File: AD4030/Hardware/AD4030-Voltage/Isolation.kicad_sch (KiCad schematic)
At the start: 23 parts, among them J401 Conn_01x08, J402 Conn_01x10, U401 ADuM260N, U402 ADuM260N

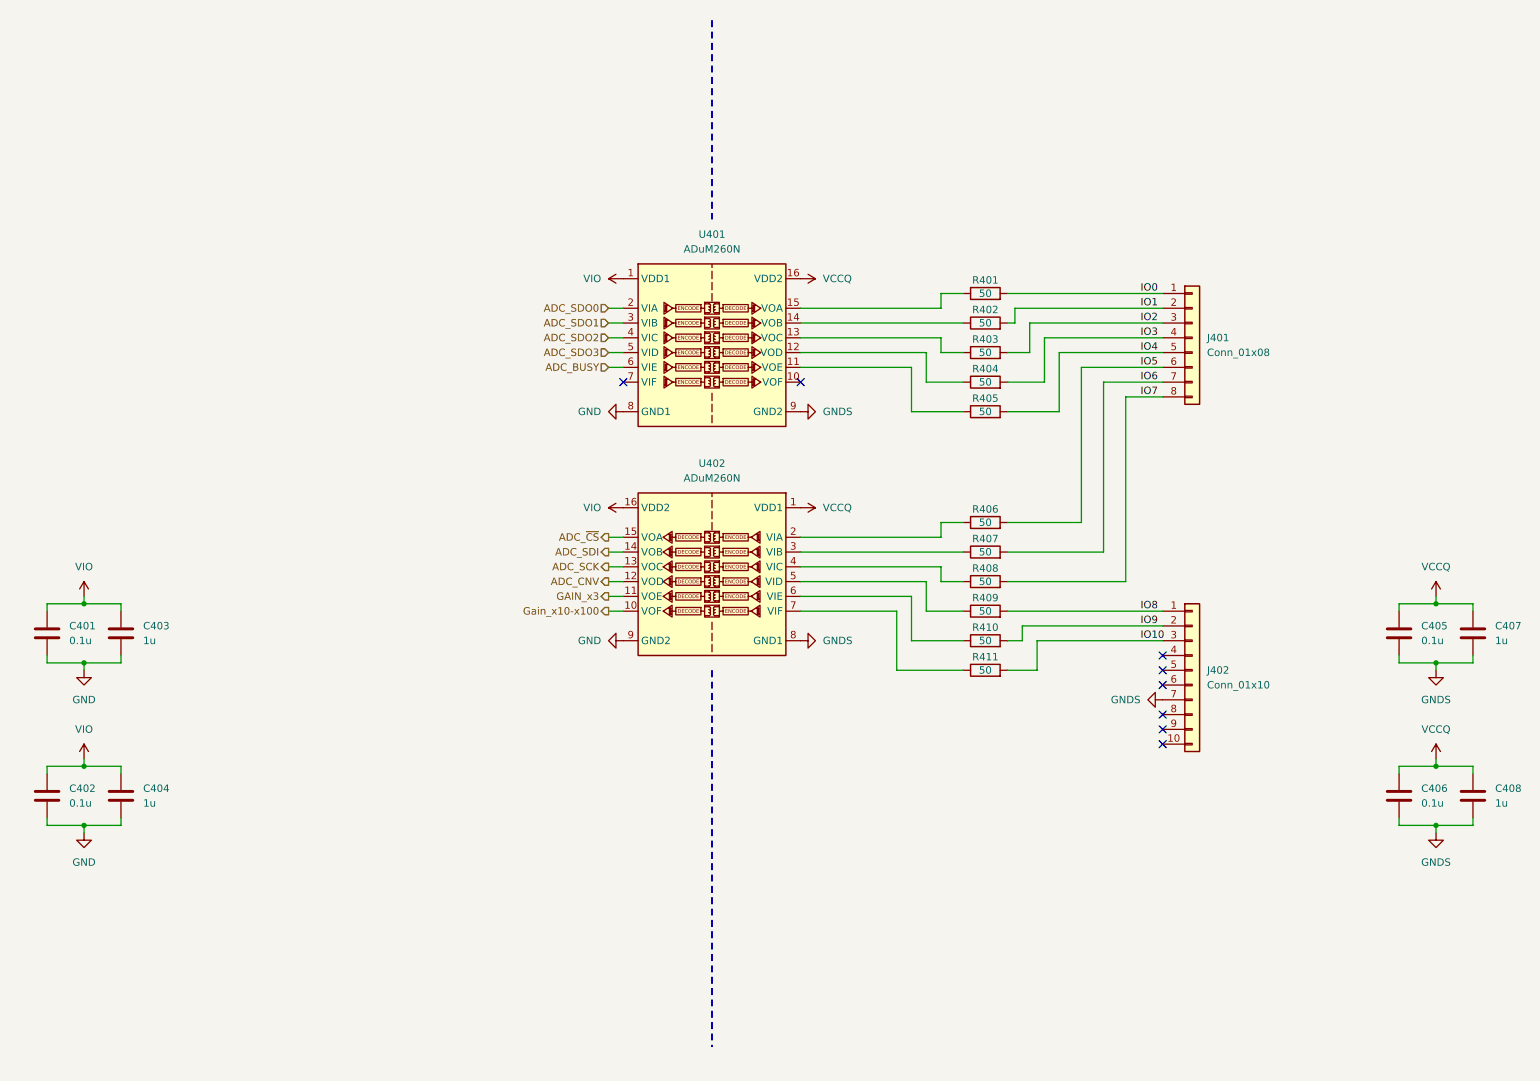
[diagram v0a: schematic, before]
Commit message: Hardware and started to create simulation.
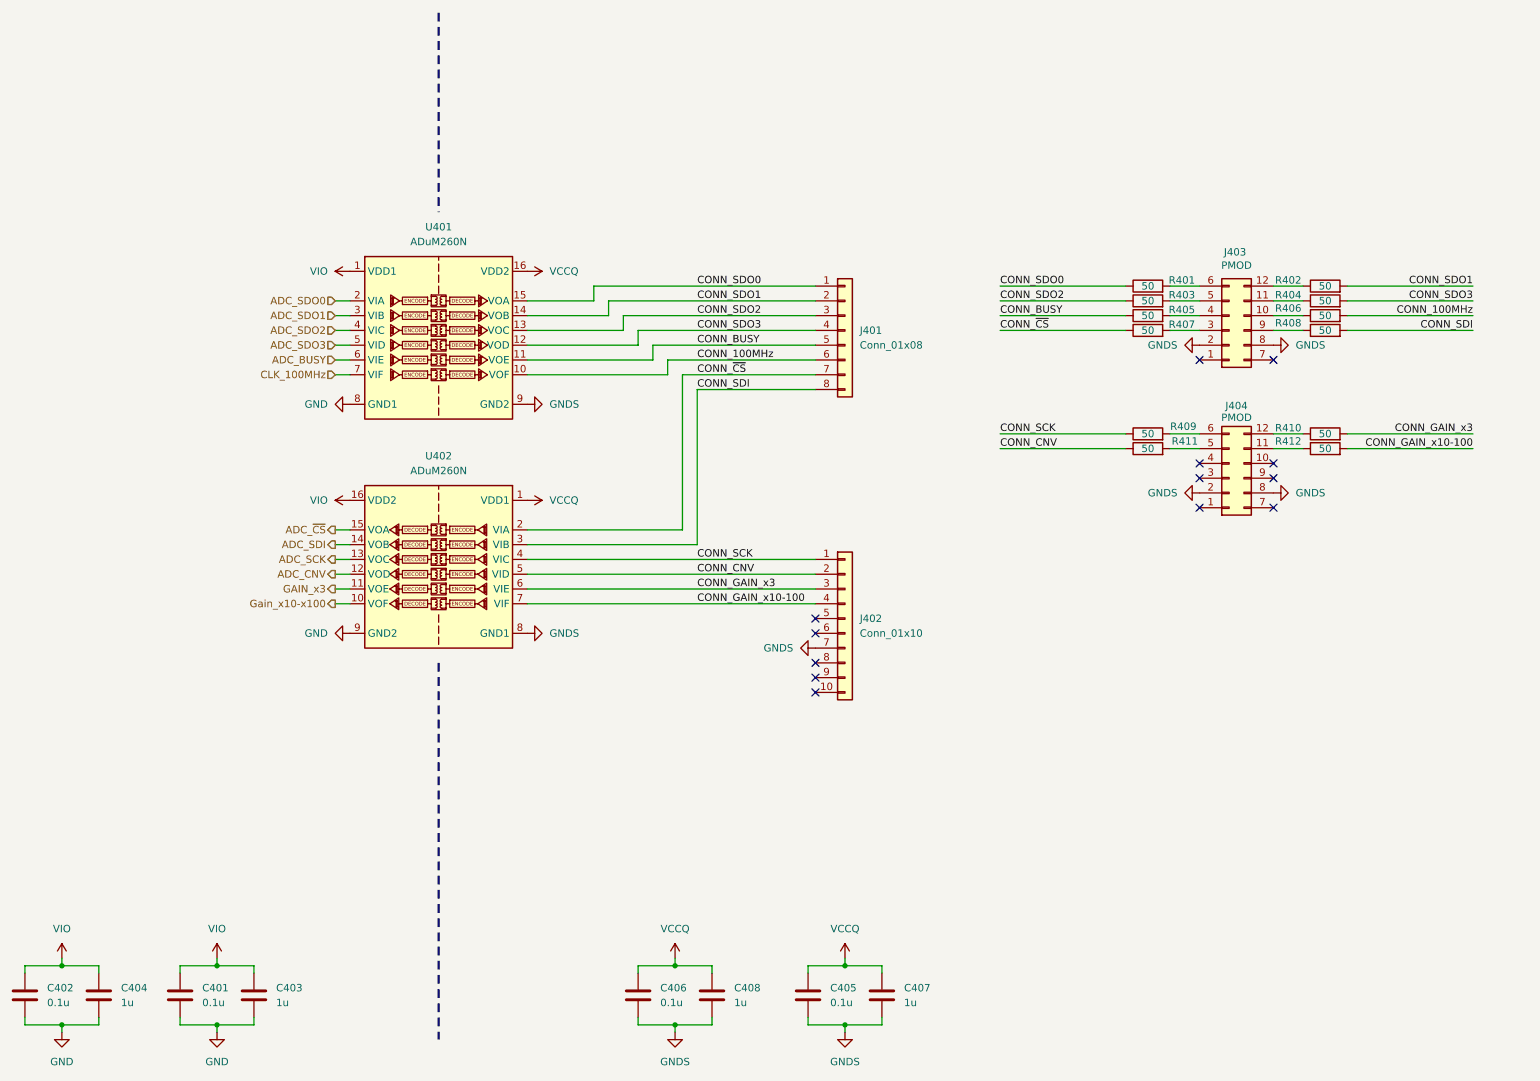
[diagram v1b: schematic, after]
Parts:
- added J403, J404: PMOD, Connector_PinHeader_2.54mm:PinHeader_2x06_P2.54mm_Horizontal, symbol Connector_Generic:Conn_02x06_Top_Bottom
- added R412: 50, Resistor_SMD:R_0603_1608Metric_Pad0.98x0.95mm_HandSolder, symbol Device:R
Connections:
- net IO5 is gone; now on net CONN_100MHz: J401.6 (Pin_6), R406.2
- net IO7 is gone; now on net CONN_SDI: J401.8 (Pin_8), R408.2
- net GNDS: now also J403.2 (Pin_2), J403.8 (Pin_8), J404.2 (Pin_2), J404.8 (Pin_8)
- net at R408.1: now also J403.9 (Pin_9); no longer U402.4 (VIC)
- net CONN_CNV: now reaches R411.1
- net CONN_CNV: now also J402.2 (Pin_2), U402.5 (VID); no longer U402.7 (VIF)
- net CONN_SDO0: now reaches R401.1, U401.15 (VOA)
- net CONN_SDO0: now also J401.1 (Pin_1)
- net at R410.1: now also J404.12 (Pin_12); no longer U402.6 (VIE)
- net CONN_SCK: now reaches R409.1
- net CONN_SCK: now also J402.1 (Pin_1), U402.4 (VIC); no longer U402.5 (VID)
- net CONN_SDO2: now reaches R403.1, U401.13 (VOC)
- net CONN_SDO2: now also J401.3 (Pin_3)
- net CONN_100MHz: now reaches U401.10 (VOF)
- net CONN_BUSY: now reaches R405.1, U401.11 (VOE)
- net CONN_BUSY: now also J401.5 (Pin_5)
- net at R404.1: now also J403.11 (Pin_11); no longer U401.12 (VOD)
- net at R402.1: now also J403.12 (Pin_12); no longer U401.14 (VOB)
- net CLK_100MHz: now reaches U401.7 (VIF)
- net CONN_SDI: now reaches U402.3 (VIB)
- net CONN_SDI: no longer R407.1
- net at R406.1: now also J403.10 (Pin_10); no longer U402.2 (VIA)
- net CONN_GAIN_x10-100: now reaches J402.4 (Pin_4)
- net CONN_GAIN_x10-100: now also U402.7 (VIF), R412.2
- net IO0: no longer names the net of R401.2
- net IO0: now also J403.6 (Pin_6); no longer J401.1 (Pin_1)
- net IO1 renamed CONN_SDO1
- net CONN_SDO1: now also U401.14 (VOB)
- net IO10: no longer names the net of R411.2
- net IO10: now also J404.5 (Pin_5); no longer J402.3 (Pin_3)
- net IO2: no longer names the net of R403.2
- net IO2: now also J403.5 (Pin_5); no longer J401.3 (Pin_3)
- net IO3 renamed CONN_SDO3
- net CONN_SDO3: now also U401.12 (VOD)
- net IO4: no longer names the net of R405.2
- net IO4: now also J403.4 (Pin_4); no longer J401.5 (Pin_5)
- net IO6: no longer names the net of R407.2
- net IO6: now also J403.3 (Pin_3); no longer J401.7 (Pin_7)
- net IO8: no longer names the net of R409.2
- net IO8: now also J404.6 (Pin_6); no longer J402.1 (Pin_1)
- net IO9 renamed CONN_GAIN_x3
- net CONN_GAIN_x3: now also J402.3 (Pin_3), U402.6 (VIE); no longer J402.2 (Pin_2)
- new net: J404.11 (Pin_11), R412.1
- new net CONN_~{CS}: J401.7 (Pin_7), R407.1, U402.2 (VIA)
- no-connect marks 8 -> 13
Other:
- moved on the sheet: C401, C402, C403, C404, C405, C406, C407, C408, J401, J402, R401, R402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
